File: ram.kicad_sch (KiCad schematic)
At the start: 7 parts, among them J12 DRAM SIMM, U13 41464, U14 41464, U17 41464, U19 41464, U20 74LS245, U21 74LS245

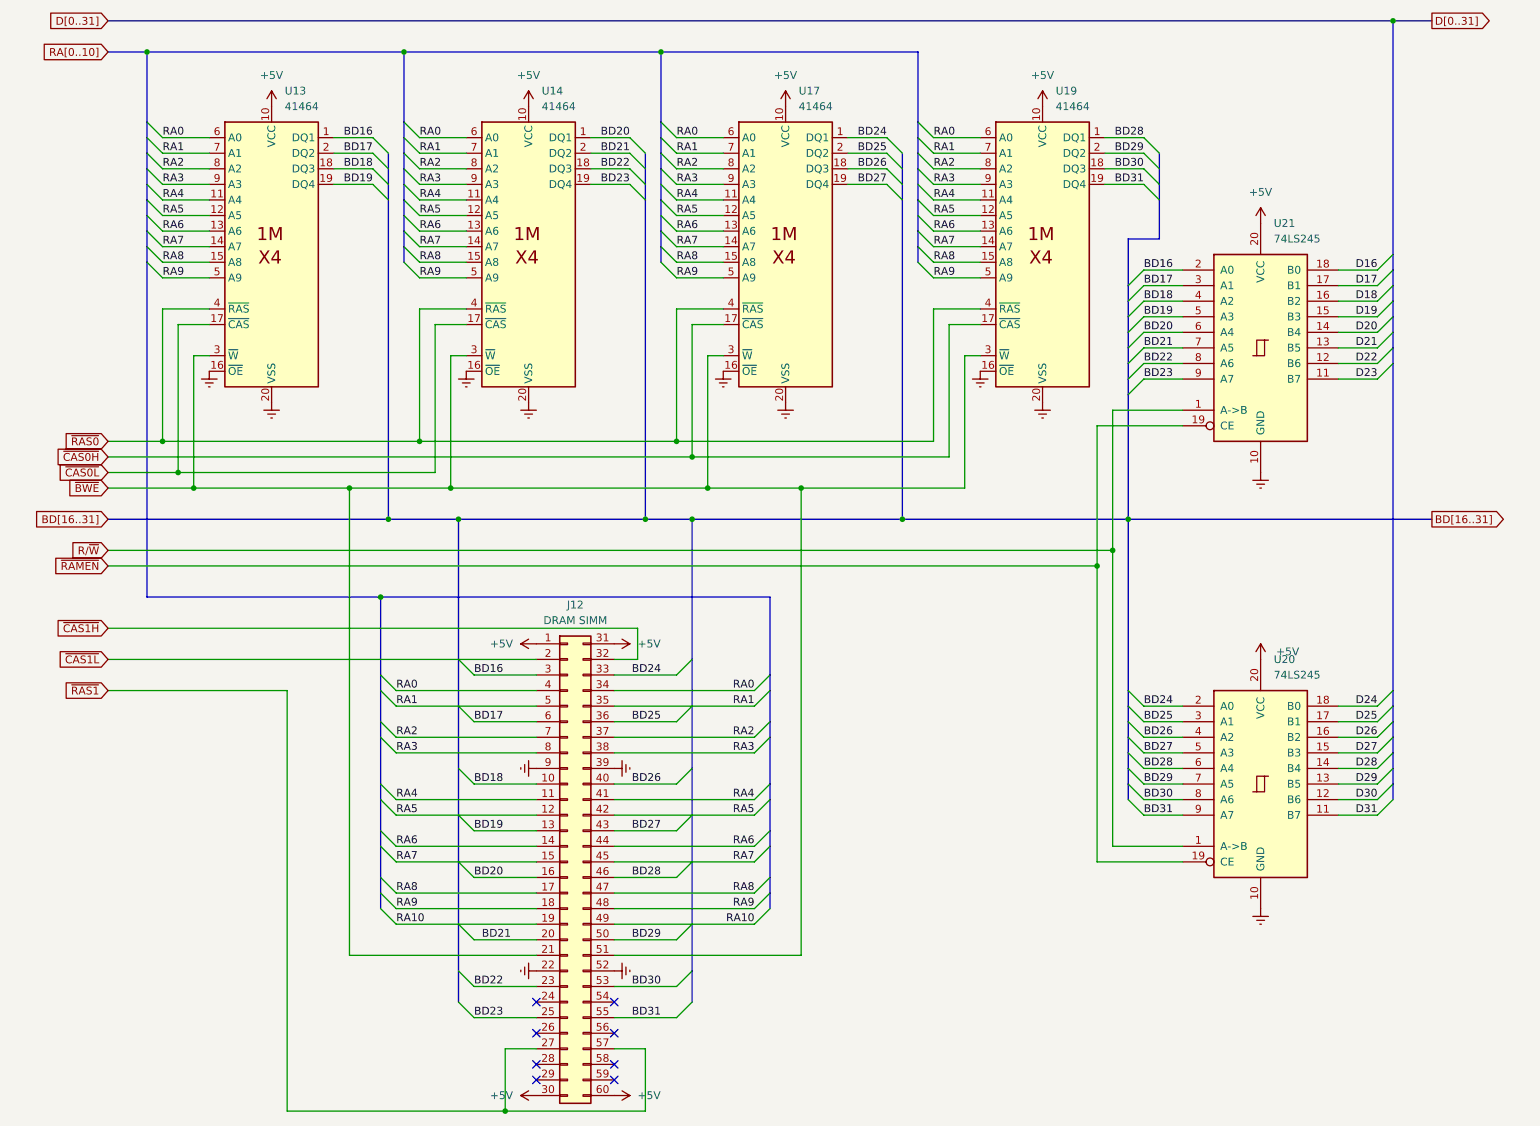
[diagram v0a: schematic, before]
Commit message: More cleanup and cosmetic fixes
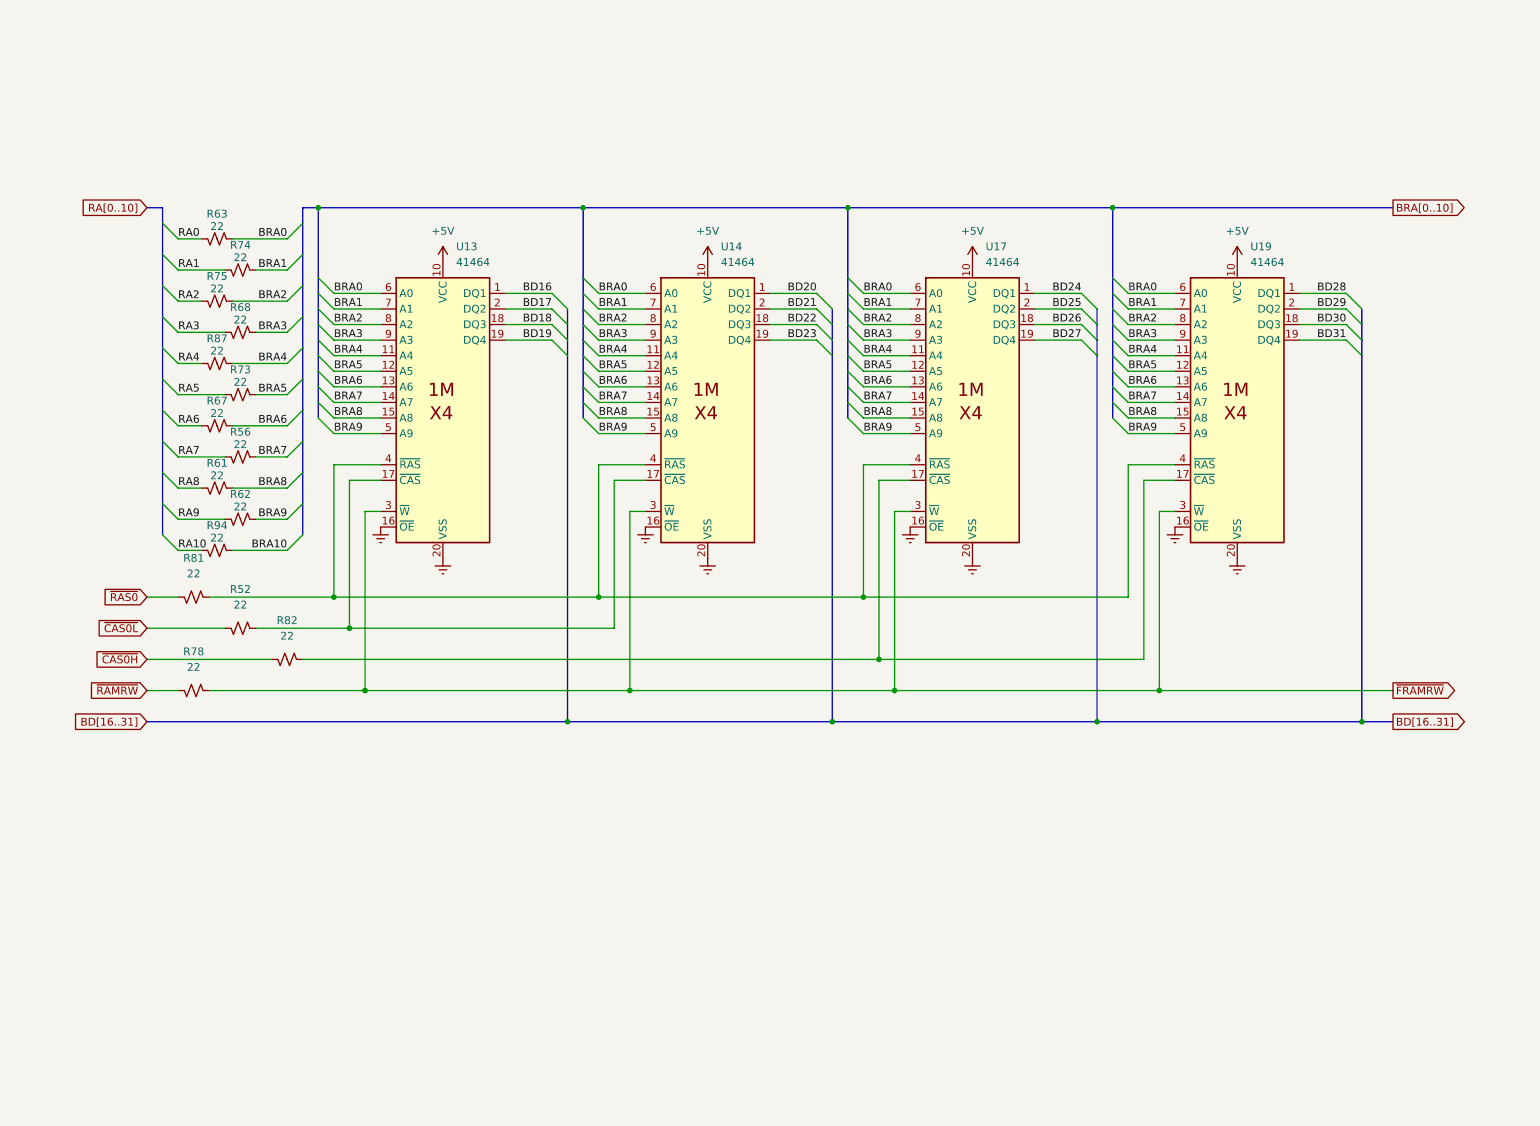
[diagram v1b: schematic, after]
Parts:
- removed J12: DRAM SIMM, Connector_Mine:SIMMSocket_2x30_angled, symbol Connector_Generic:Conn_02x30_Top_Bottom
- removed U20, U21: 74LS245, MyPackage:SOIC-20W_7.5x12.8mm_P1.27mm_oval, symbol 74xx:74LS245
- added R52, R56, R61, R62, R63, R67, R68, R73, R74, R75, R78, R81, R82, R87, R94: 22, MyPackage:SMD_0805_2012Metric_Pad1.25x1.65mm, symbol Device:R_Small_US
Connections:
- net RA0: now also R63.2; no longer U13.6 (A0), U14.6 (A0), U17.6 (A0), U19.6 (A0)
- net RA1: now also R74.2; no longer U13.7 (A1), U14.7 (A1), U17.7 (A1), U19.7 (A1)
- net RA10: now also R94.1
- net RA2: now also R75.2; no longer U13.8 (A2), U14.8 (A2), U17.8 (A2), U19.8 (A2)
- net RA3: now also R68.2; no longer U13.9 (A3), U14.9 (A3), U17.9 (A3), U19.9 (A3)
- net RA4: now also R87.2; no longer U13.11 (A4), U14.11 (A4), U17.11 (A4), U19.11 (A4)
- net RA5: now also R73.1; no longer U13.12 (A5), U14.12 (A5), U17.12 (A5), U19.12 (A5)
- net RA6: now also R67.1; no longer U13.13 (A6), U14.13 (A6), U17.13 (A6), U19.13 (A6)
- net RA7: now also R56.1; no longer U13.14 (A7), U14.14 (A7), U17.14 (A7), U19.14 (A7)
- net RA8: now also R61.1; no longer U13.15 (A8), U14.15 (A8), U17.15 (A8), U19.15 (A8)
- net RA9: now also R62.1; no longer U13.5 (A9), U14.5 (A9), U17.5 (A9), U19.5 (A9)
- net ~{CAS0H}: now also R82.1; no longer U17.17 (~{CAS}), U19.17 (~{CAS})
- net ~{CAS0L}: now also R52.1; no longer U13.17 (~{CAS}), U14.17 (~{CAS})
- net ~{RAS0}: now also R81.2; no longer U13.4 (~{RAS}), U14.4 (~{RAS}), U17.4 (~{RAS}), U19.4 (~{RAS})
- net ~{BWE} renamed ~{FRAMRW}
- net ~{FRAMRW}: now also R78.1
- new net: R81.1, U13.4 (~{RAS}), U14.4 (~{RAS}), U17.4 (~{RAS}), U19.4 (~{RAS})
- new net: R52.2, U13.17 (~{CAS}), U14.17 (~{CAS})
- new net: R82.2, U17.17 (~{CAS}), U19.17 (~{CAS})
- new net BRA0: R63.1, U13.6 (A0), U14.6 (A0), U17.6 (A0), U19.6 (A0)
- new net BRA1: R74.1, U13.7 (A1), U14.7 (A1), U17.7 (A1), U19.7 (A1)
- new net BRA10: R94.2
- new net BRA2: R75.1, U13.8 (A2), U14.8 (A2), U17.8 (A2), U19.8 (A2)
- new net BRA3: R68.1, U13.9 (A3), U14.9 (A3), U17.9 (A3), U19.9 (A3)
- new net BRA4: R87.1, U13.11 (A4), U14.11 (A4), U17.11 (A4), U19.11 (A4)
- new net BRA5: R73.2, U13.12 (A5), U14.12 (A5), U17.12 (A5), U19.12 (A5)
- new net BRA6: R67.2, U13.13 (A6), U14.13 (A6), U17.13 (A6), U19.13 (A6)
- new net BRA7: R56.2, U13.14 (A7), U14.14 (A7), U17.14 (A7), U19.14 (A7)
- new net BRA8: R61.2, U13.15 (A8), U14.15 (A8), U17.15 (A8), U19.15 (A8)
- new net BRA9: R62.2, U13.5 (A9), U14.5 (A9), U17.5 (A9), U19.5 (A9)
- new net ~{RAMRW}: R78.2
- no-connect marks 8 -> 0
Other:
- moved on the sheet: U13, U14, U17, U19
